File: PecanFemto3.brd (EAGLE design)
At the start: 28.9 x 10.2 mm, 31 parts, among them U1 TPS62203DBVT

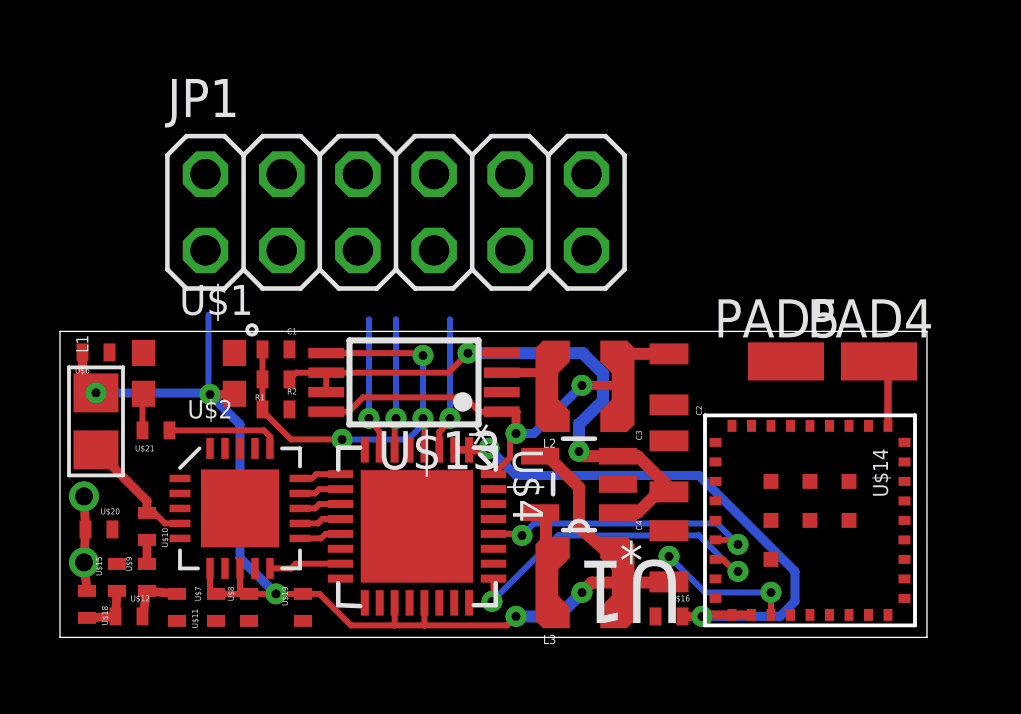
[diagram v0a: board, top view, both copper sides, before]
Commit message: Routed parts
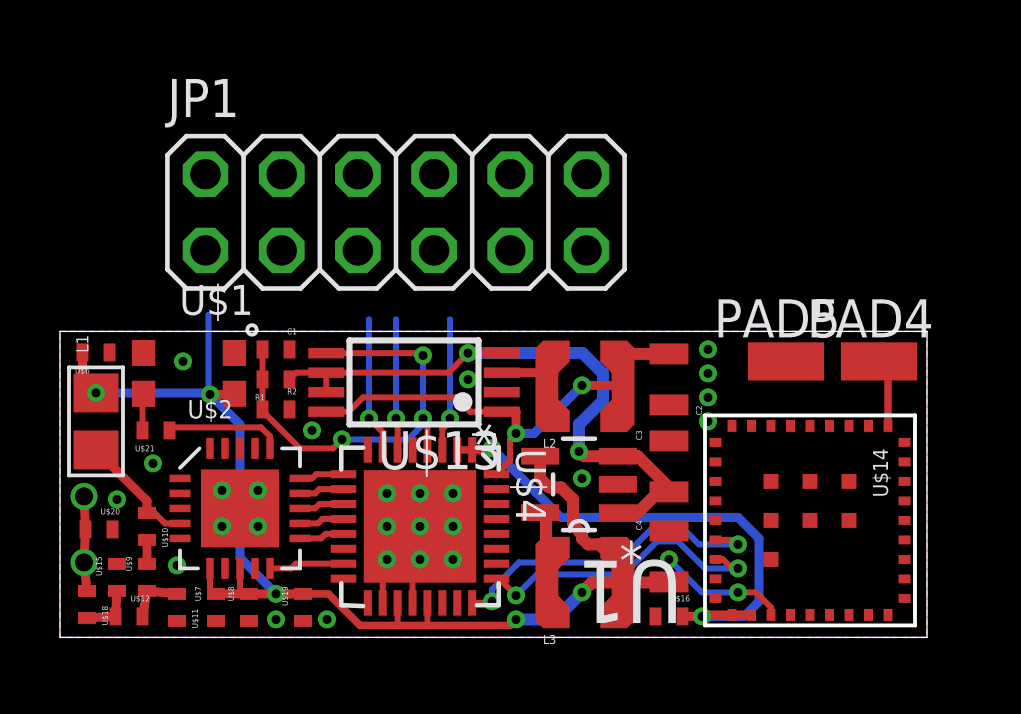
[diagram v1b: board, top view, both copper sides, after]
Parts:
- moved U$4 0.10 mm to (26.5, 18.7)
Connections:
- net RXD: now also U$4.24; no longer U$4.28
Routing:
- net GND: track 0.00 -> 4.74 mm, vias 0 -> 26
- net VCC_GPS: track 19.7 -> 17.8 mm
- net RXD: track 9.44 -> 11.1 mm
- net TXD: track 11.3 -> 10.4 mm
- added copper zone on layer 1, net GND
- added copper zone on layer 16, net GND
